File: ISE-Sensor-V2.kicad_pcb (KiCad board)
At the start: 4 copper layers, 17 x 45.8 mm, 45 parts, among them CN1 BM04B-SRSS-TB(LF)(SN), U12 ADS122C04IRTER, U14 OPA928, U16 TPS7A2025PDBVR, U17 LM2776, U18 TPS72325DBV, U5 ADM3260

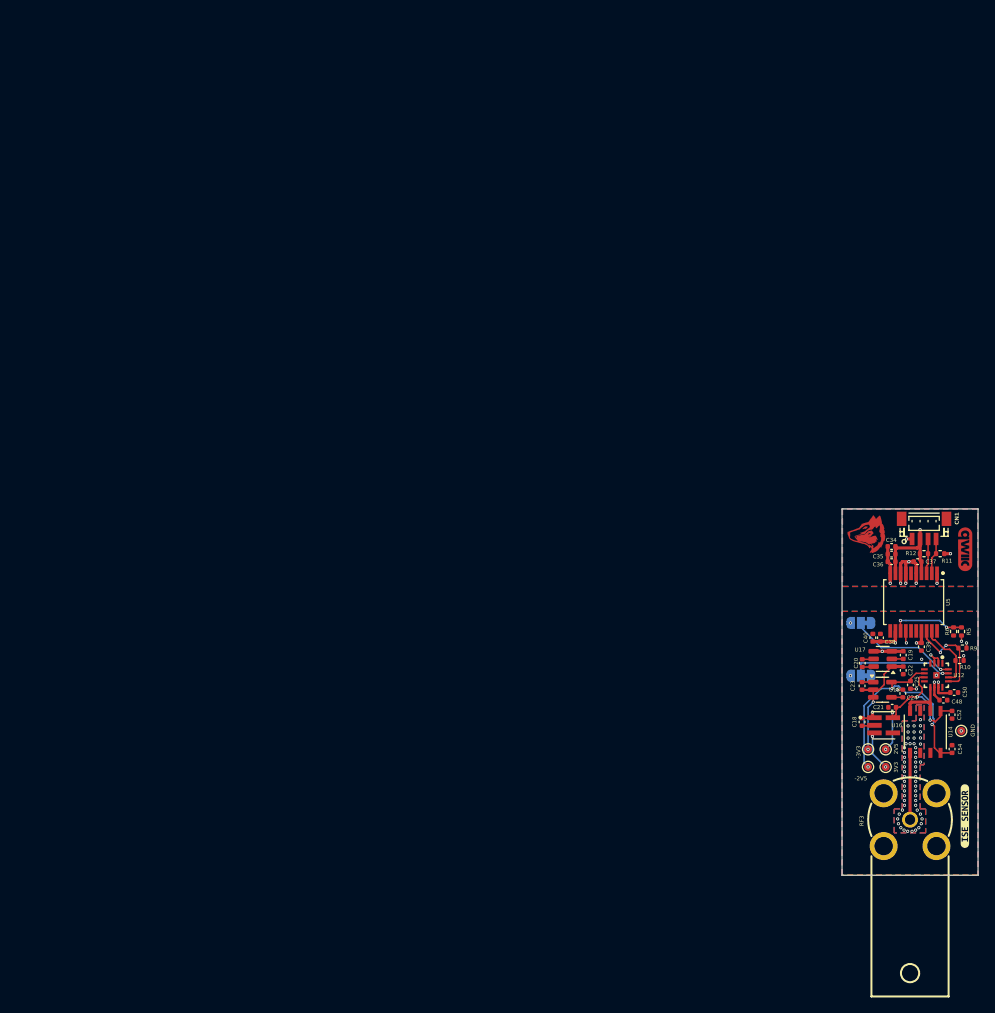
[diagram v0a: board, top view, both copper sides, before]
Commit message: Update images
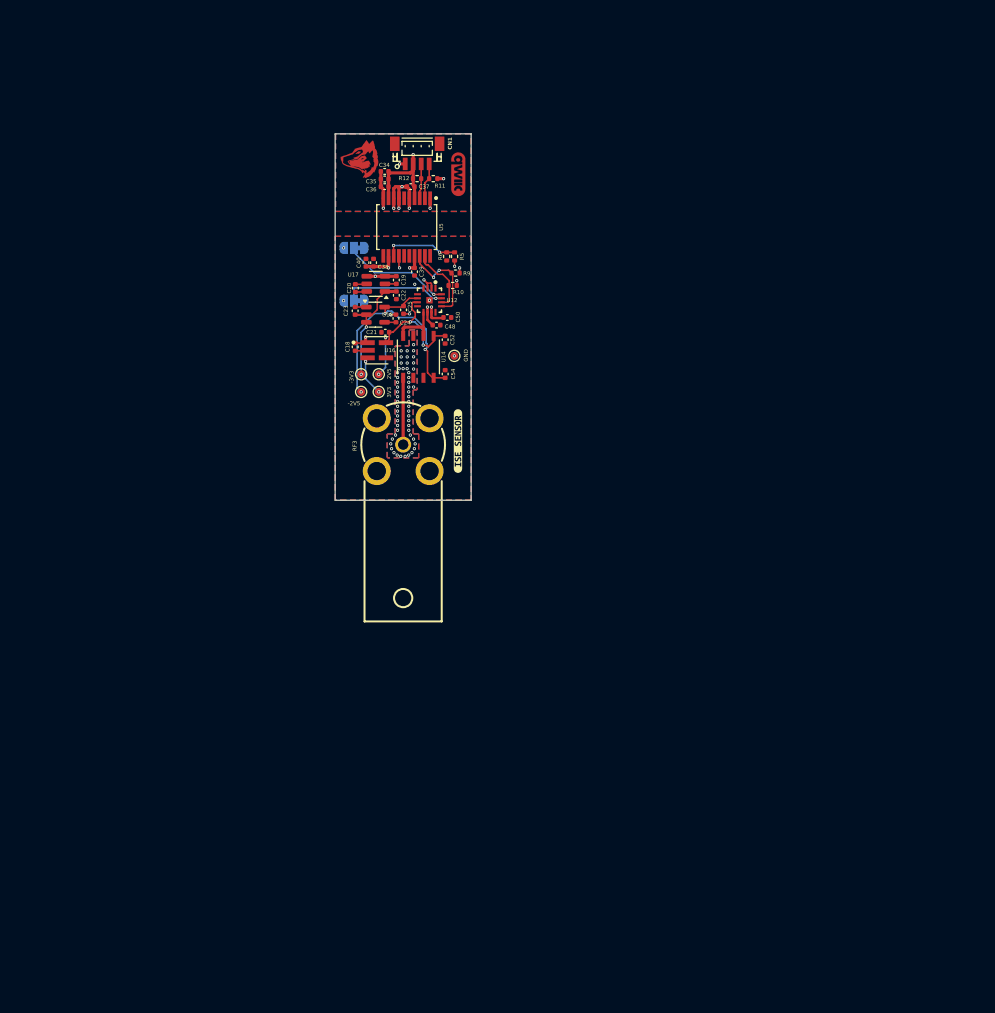
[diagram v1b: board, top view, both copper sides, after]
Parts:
- moved C34 78.8 mm to (66.1, 34.4)
- moved C35 78.8 mm to (66.1, 35.4)
- moved C36 78.8 mm to (66.1, 36.3)
- moved C37 78.8 mm to (69.3, 36.3)
- moved C40 78.8 mm to (63.7, 45.8)
- moved C52 78.8 mm to (73.6, 55.5)
- moved C54 78.8 mm to (73.6, 59.7)
- moved G*** 78.8 mm to (75.3, 34.8)
- moved R10 78.8 mm to (74.6, 48.7)
- moved R12 78.8 mm to (70.1, 35.3)
- moved R6 78.8 mm to (73.8, 45.0)
- moved C18 78.8 mm to (62.4, 56.4)
- moved C20 78.8 mm to (62.4, 49.0)
- moved C23 78.8 mm to (62.4, 51.8)
- moved C24 78.8 mm to (67.5, 52.8)
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
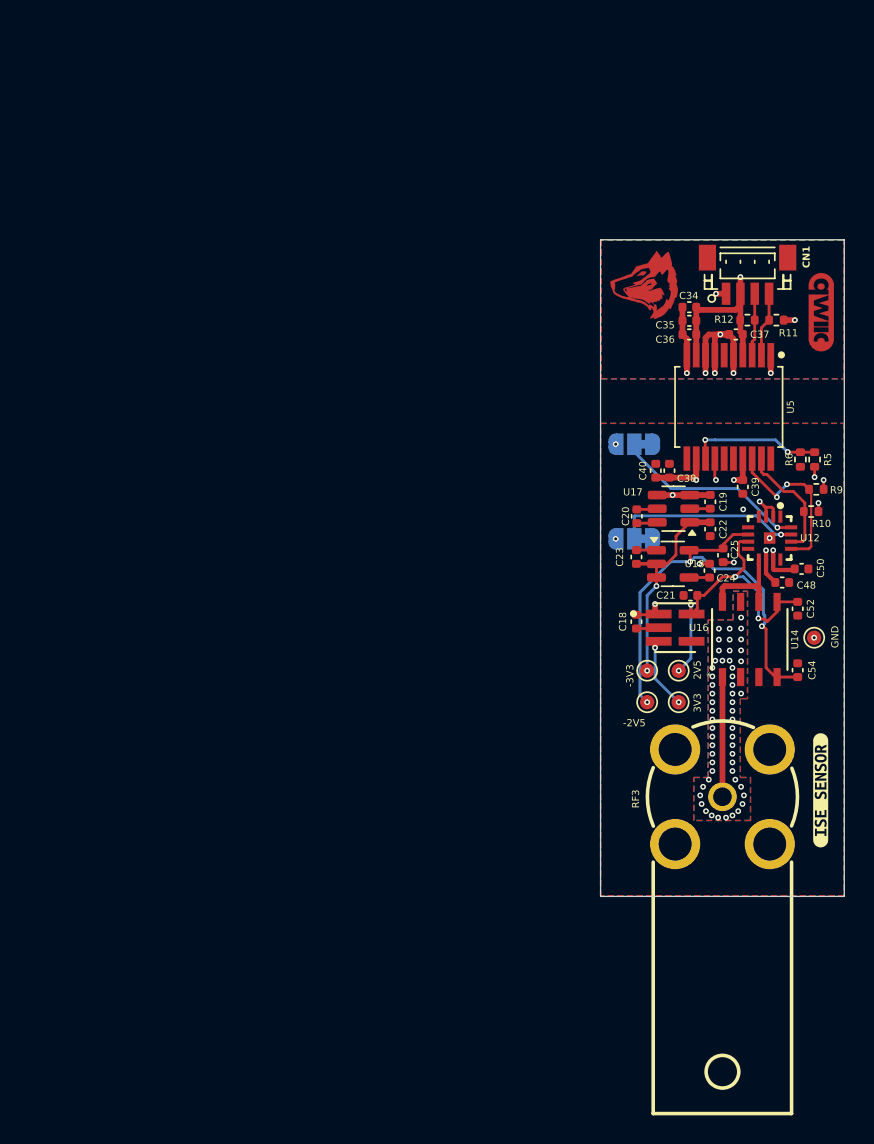
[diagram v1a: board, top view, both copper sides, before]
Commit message: Updates
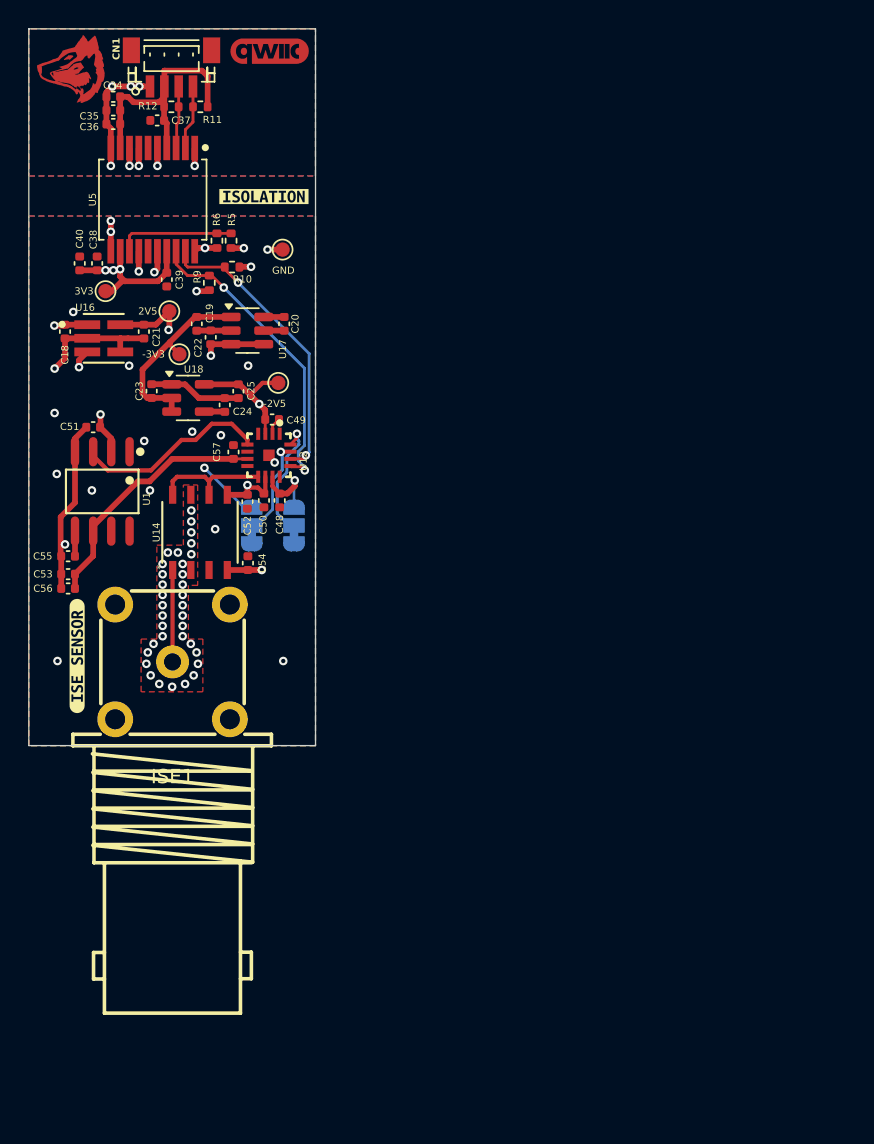
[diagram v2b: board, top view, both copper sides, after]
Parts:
- removed RF3: ORP Sensor, EasyEDA:BNC-TH_DOSIN-801-0051
- added C49: 100nF, Capacitor_SMD:C_0402_1005Metric, F.Cu at (37.0, 42.2)
- added C51: 10uF, Capacitor_SMD:C_0402_1005Metric, F.Cu at (24.5, 42.8)
- added C53: 50uF, Capacitor_SMD:C_0402_1005Metric, F.Cu at (22.7, 53.0)
- added C55: 1uF, Capacitor_SMD:C_0402_1005Metric, F.Cu at (22.7, 51.8)
- added C56: 1uF, Capacitor_SMD:C_0402_1005Metric, F.Cu at (22.7, 54.0)
- added C57: 100nF, Capacitor_SMD:C_0402_1005Metric, F.Cu at (34.3, 44.5)
- added ISE1: DOSIN-801-0080, EasyEDA:BNC-TH_DOSIN-801-0080, F.Cu at (30.0, 59.2)
- added U1: REF5025IDR, EasyEDA:SOIC-8_L4.9-W3.9-P1.27-LS6.0-BL, F.Cu at (25.1, 47.3)
- added kibuzzard-67B4F71A: G***, kibuzzard-67B4F71A, F.Cu at (36.4, 26.7)
- moved kibuzzard-67AA55DF 52.7 mm to (23.4, 58.8)
- moved TP6 49.2 mm to (25.4, 33.3), turned to -90 degrees
- moved TP12 45.9 mm to (37.7, 30.4), turned to -90 degrees
- moved R9 44.7 mm to (32.6, 32.7), turned to 90 degrees
- moved C18 44.7 mm to (22.5, 36.1)
- moved U16 44.7 mm to (25.2, 36.6)
- moved R10 43.8 mm to (34.2, 31.6)
- moved TP10 43.5 mm to (29.8, 34.7), turned to -90 degrees
- moved R5 43.5 mm to (34.1, 29.8)
- moved R6 43.5 mm to (33.1, 29.8)
- moved C37 43.0 mm to (29.0, 21.4)
- moved R11 42.9 mm to (32.0, 20.4)
- moved R12 42.9 mm to (29.9, 20.4)
- moved C34 42.8 mm to (25.9, 19.7)
- moved C35 42.8 mm to (25.9, 20.7)
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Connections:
- net /ORP/ISO_-3V3 renamed /ORP/PP_ISO_NEG_3V3
- C18 pad 1: /ISO_3V3 -> /PP_ISO_3V3
- C19 pad 1: /ISO_3V3 -> /PP_ISO_3V3
- C21 pad 1: /ORP/ISO_2V5 -> /ORP/PP_ISO_2V5
- C25 pad 2: /ORP/ISO_-2V5 -> /ORP/PP_ISO_NEG_2V5
- C38 pad 1: /ISO_3V3 -> /PP_ISO_3V3
- C39 pad 1: /ISO_3V3 -> /PP_ISO_3V3
- C40 pad 1: /ISO_3V3 -> /PP_ISO_3V3
- C48 pad 1: /ISO_3V3 -> /PP_ISO_3V3
- C50 pad 1: /ISO_3V3 -> /ORP/PP_ISO_2V5
- C52 pad 2: /ORP/ISO_2V5 -> /ORP/PP_ISO_2V5
- C54 pad 2: /ORP/ISO_-2V5 -> /ORP/PP_ISO_NEG_2V5
- JP3 pad 3: /ISO_3V3 -> /PP_ISO_3V3
- JP4 pad 3: /ISO_3V3 -> /PP_ISO_3V3
- R10 pad 2: /ISO_3V3 -> /PP_ISO_3V3
- R5 pad 2: /ISO_3V3 -> /PP_ISO_3V3
- R9 pad 1: /ISO_3V3 -> /PP_ISO_3V3
- TP10 pad 1: /ORP/ISO_2V5 -> /ORP/PP_ISO_2V5
- TP11 pad 1: /ORP/ISO_-2V5 -> /ORP/PP_ISO_NEG_2V5
- TP6 pad 1: /ISO_3V3 -> /PP_ISO_3V3
- U12 pad 10: /ISO_3V3 -> /ORP/PP_ISO_2V5
- U12 pad 11: /ISO_3V3 -> /PP_ISO_3V3
- U12 pad 3: /ISO_GND -> /ORP/PP_ISO_NEG_2V5
- U12 pad 5: unconnected-(U12-AIN2-Pad5) -> /ORP/TEMP
- U12 pad 6: /ORP/ISO_-2V5 -> unconnected-(U12-REFN-Pad6)
- U12 pad 7: /ORP/ISO_2V5 -> /ORP/PP_ISO_REF_2V5
- U14 pad 4: /ORP/ISO_-2V5 -> /ORP/PP_ISO_NEG_2V5
- U14 pad 5: /ORP/ISO_2V5 -> /ORP/PP_ISO_2V5
- U16 pad 1: /ISO_3V3 -> /PP_ISO_3V3
- U16 pad 3: /ISO_3V3 -> /PP_ISO_3V3
- U16 pad 5: /ORP/ISO_2V5 -> /ORP/PP_ISO_2V5
- U17 pad 3: /ISO_3V3 -> /PP_ISO_3V3
- U17 pad 4: /ISO_3V3 -> /PP_ISO_3V3
- U18 pad 5: /ORP/ISO_-2V5 -> /ORP/PP_ISO_NEG_2V5
- U5 pad 12: /ISO_3V3 -> /PP_ISO_3V3
- U5 pad 17: /ISO_3V3 -> /PP_ISO_3V3
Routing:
- net /PP_ISO_3V3: track 0.00 -> 34.2 mm, vias 0 -> 12
- net /ORP/ISO_-2V5: track 32.2 -> 0.00 mm, vias 3 -> 0
- net /ISO_GND: track 9.82 -> 38.7 mm, vias 7 -> 22
- net /ISO_3V3: track 25.7 -> 0.00 mm, vias 13 -> 0
- net /ORP/PP_ISO_2V5: track 0.00 -> 23.0 mm, vias 0 -> 2
- net /ORP/PP_ISO_NEG_2V5: track 0.00 -> 23.0 mm, vias 0 -> 2
- net /ORP/ISO_2V5: track 21.4 -> 0.00 mm, vias 4 -> 0
- net /ORP/PP_ISO_REF_2V5: track 0.00 -> 17.6 mm
- net /ORP/TEMP: track 0.00 -> 13.6 mm
- net /ORP/ISO_SCL: track 8.43 -> 20.7 mm, vias 0 -> 2
- net /ORP/ISO_SDA: track 12.0 -> 21.5 mm
- net /A0: track 13.1 -> 6.25 mm
- net /A1: track 13.7 -> 8.70 mm
- net GND: track 17.3 -> 13.5 mm, vias 7 -> 8
- net /ORP/PP_ISO_NEG_3V3: track 16.2 -> 13.6 mm, vias 2 -> 0
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- added copper zone on In2.Cu, net /PP_ISO_3V3
- removed copper zone on In2.Cu, net /ISO_3V3
- removed copper zone on B.Cu, net /ORP/GRD
- removed copper zone on In2.Cu, net /ORP/GRD
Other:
- board size 17 x 45.8 mm -> 20 x 50 mm
